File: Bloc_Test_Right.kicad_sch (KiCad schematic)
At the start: 44 parts, among them Q29 2N7000, Q30 2N7000, Q31 2N7000, Q32 2N7000, Q33 2N7000, Q34 2N7000

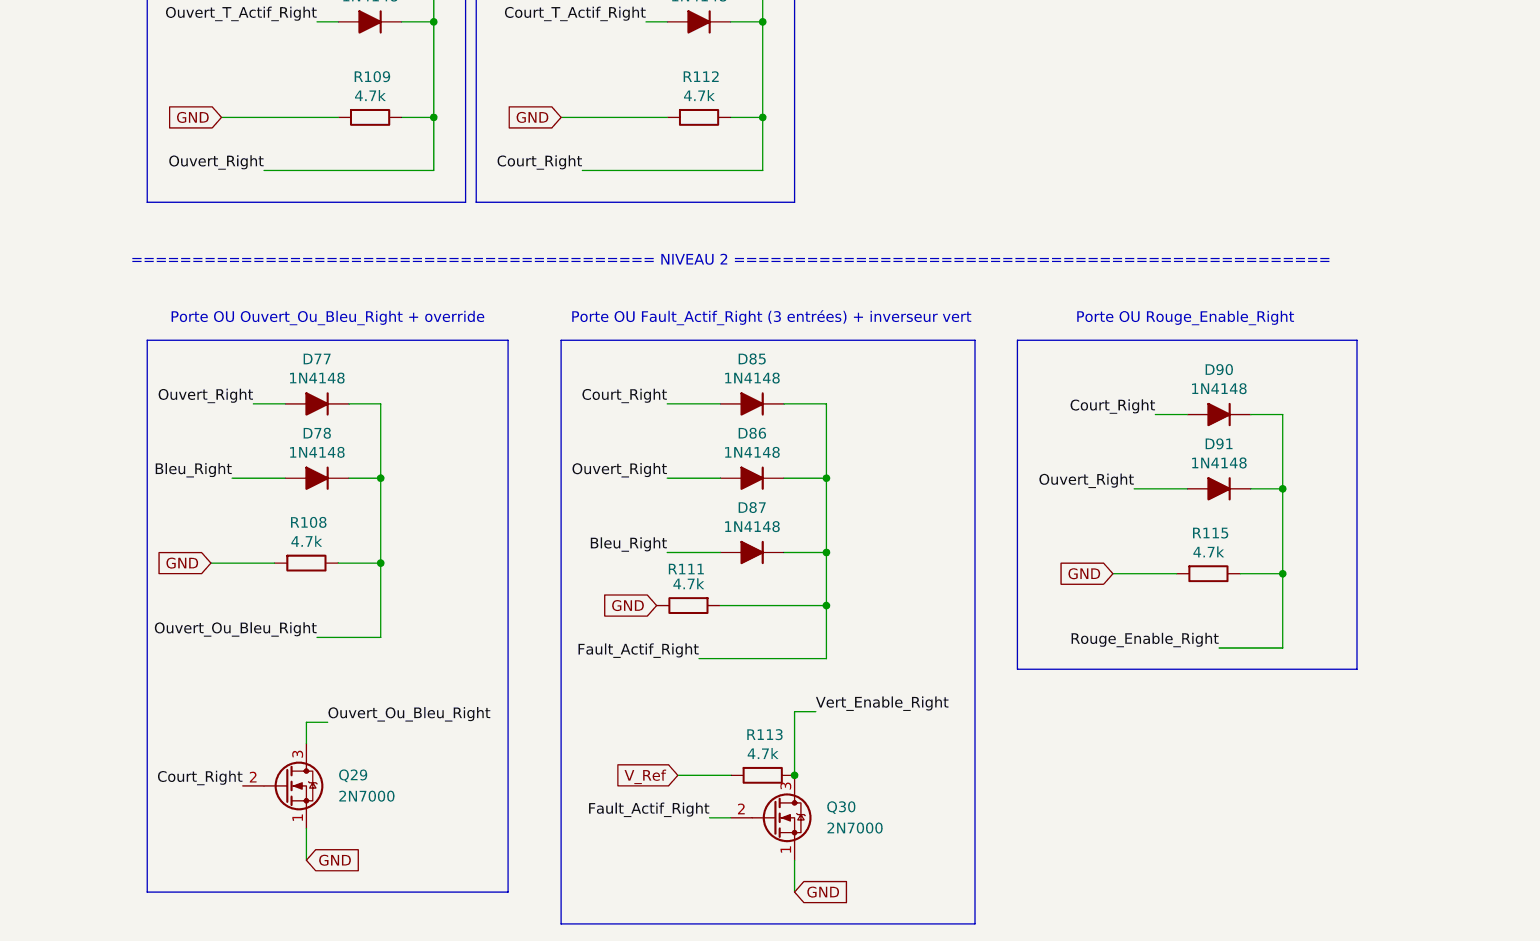
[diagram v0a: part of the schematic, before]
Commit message: Add files via upload
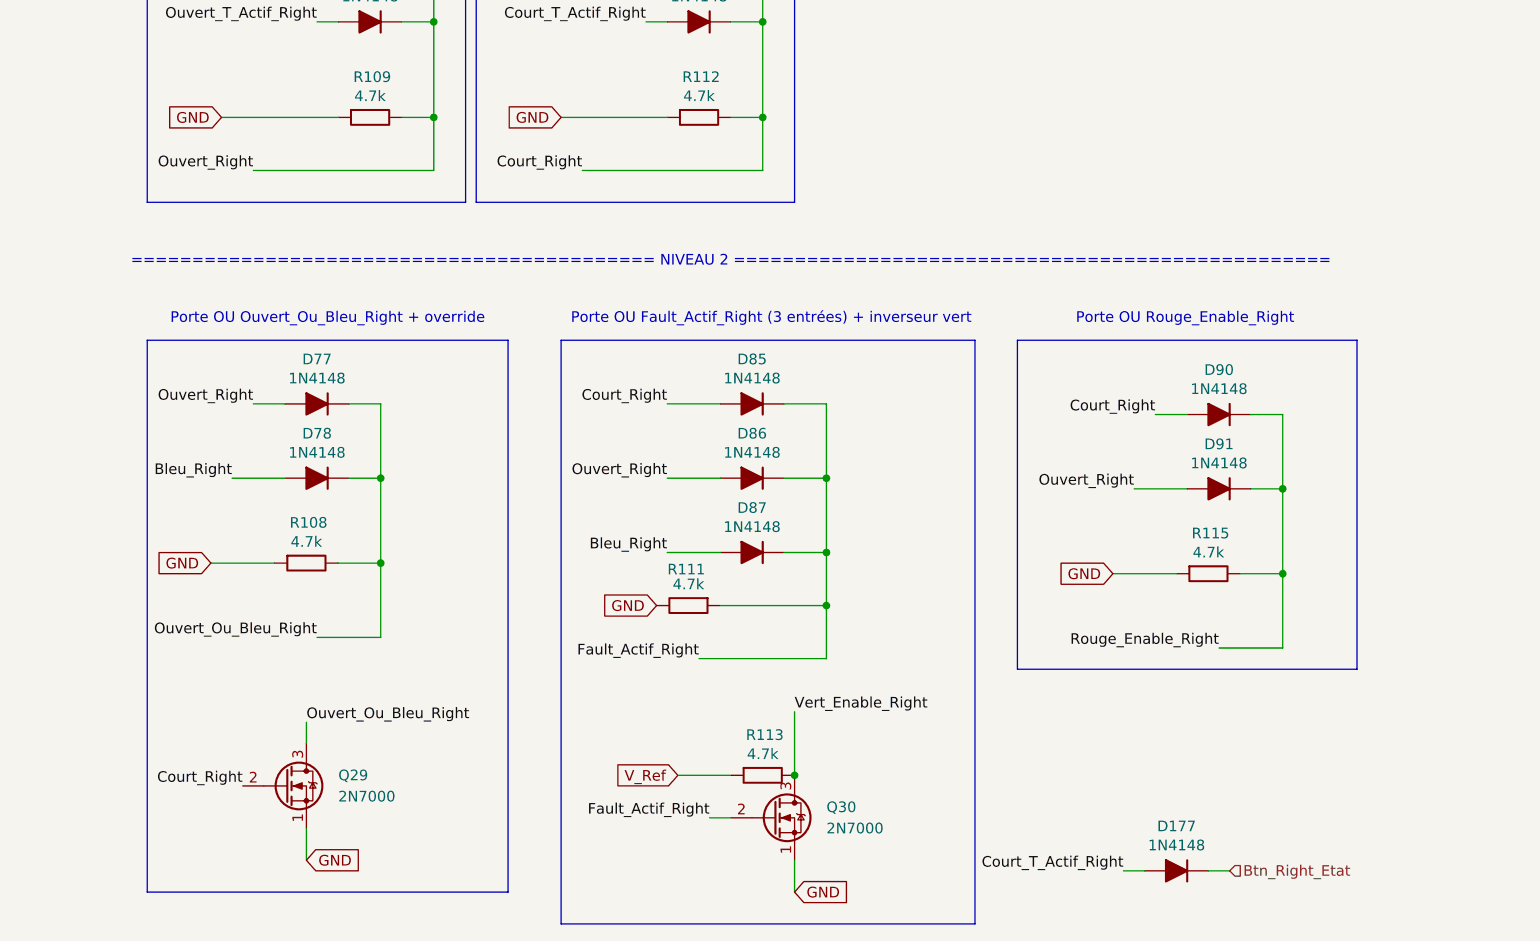
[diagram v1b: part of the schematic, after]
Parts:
- added D177: 1N4148, PCM_Diode_THT_AKL:D_DO-35_SOD27_P7.62mm_Horizontal, symbol PCM_Diode_AKL:1N4148
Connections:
- net Btn_Right_Etat: now also D177.1 (K)
- net Court_T_Actif_Right: now also D177.2 (A)

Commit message: Add files via upload
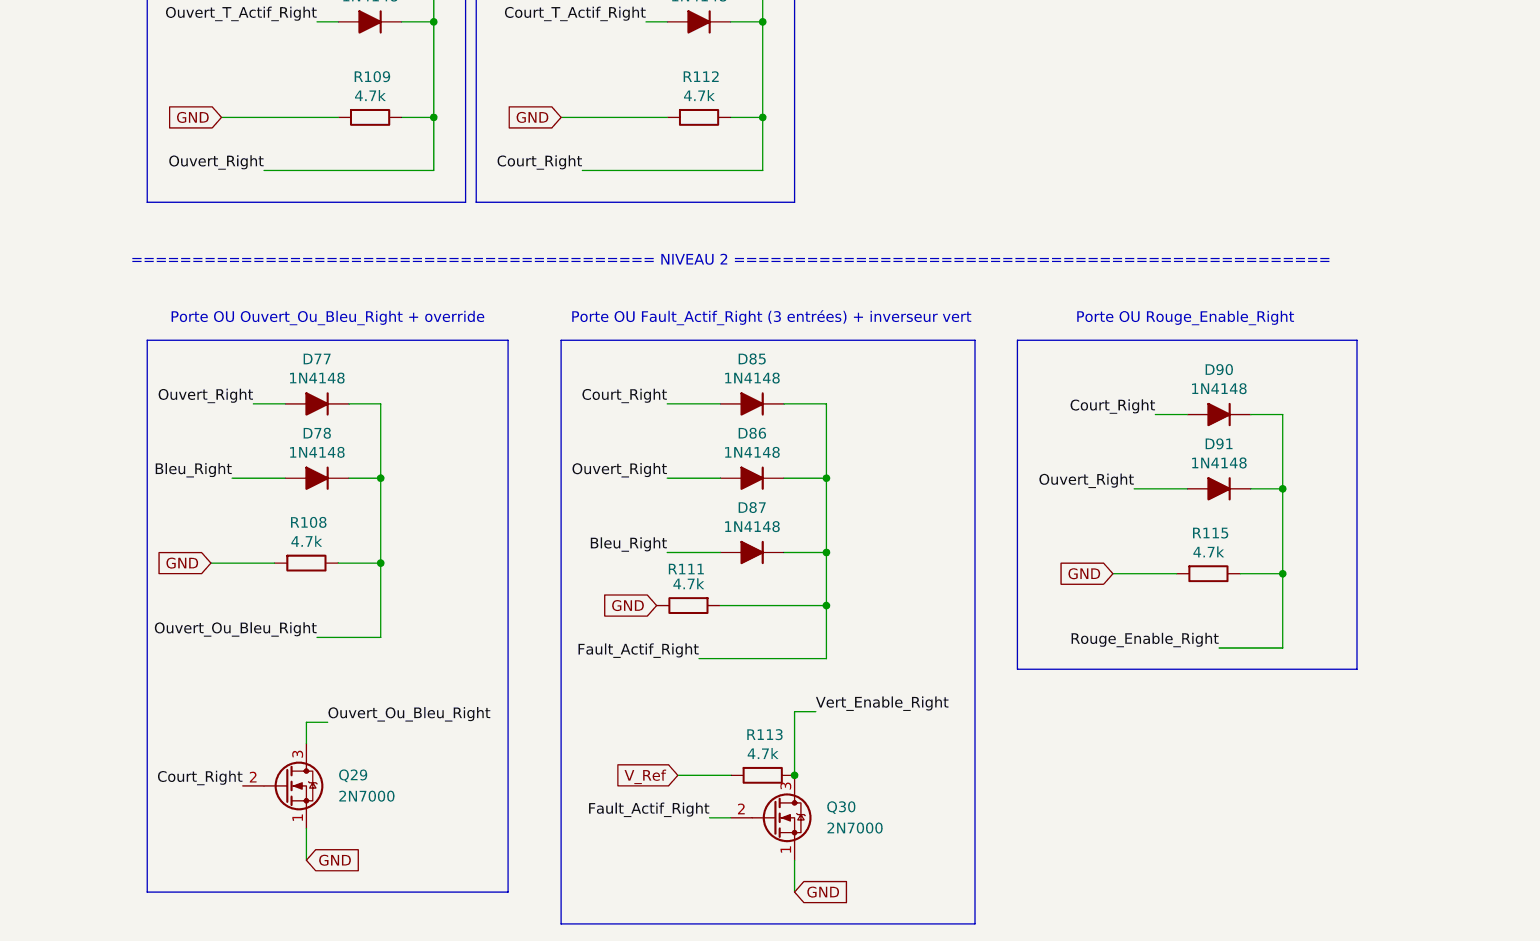
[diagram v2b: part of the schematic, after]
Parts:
- removed D177: 1N4148, PCM_Diode_THT_AKL:D_DO-35_SOD27_P7.62mm_Horizontal, symbol PCM_Diode_AKL:1N4148
